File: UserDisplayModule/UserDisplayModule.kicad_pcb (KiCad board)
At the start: 2 copper layers, 0 parts

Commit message: doubled LEDs + started PCB
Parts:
- added C1: 10µ, Capacitor_SMD:C_0805_2012Metric, F.Cu at (60.5, 129.8)
- added D1: MAINS, LED_SMD:LED_0805_2012Metric, F.Cu at (89.2, 78.9)
- added D10: BAT3, LED_SMD:LED_0805_2012Metric, F.Cu at (93.7, 91.1)
- added D11: BAT8, LED_SMD:LED_0805_2012Metric, F.Cu at (100.0, 41.8)
- added D12: BAT1, LED_SMD:LED_0805_2012Metric, F.Cu at (100.0, 44.9)
- added D13: BAT7, LED_SMD:LED_0805_2012Metric, F.Cu at (100.0, 47.9)
- added D14: BAT1, LED_SMD:LED_0805_2012Metric, F.Cu at (100.0, 51.0)
- added D15: BAT6, LED_SMD:LED_0805_2012Metric, F.Cu at (104.5, 41.8)
- added D16: BAT1, LED_SMD:LED_0805_2012Metric, F.Cu at (104.5, 44.9)
- added D17: BAT5, LED_SMD:LED_0805_2012Metric, F.Cu at (104.5, 47.9)
- added D18: BAT1, LED_SMD:LED_0805_2012Metric, F.Cu at (104.5, 51.0)
- added D19: BAT4, LED_SMD:LED_0805_2012Metric, F.Cu at (108.9, 41.8)
- added D2: MAINS, LED_SMD:LED_0805_2012Metric, F.Cu at (89.2, 82.0)
- added D20: BAT1, LED_SMD:LED_0805_2012Metric, F.Cu at (108.9, 44.9)
- added D21: BAT3, LED_SMD:LED_0805_2012Metric, F.Cu at (108.9, 47.9)
- added D22: BAT1, LED_SMD:LED_0805_2012Metric, F.Cu at (108.9, 51.0)
- added D23: BAT2, LED_SMD:LED_0805_2012Metric, F.Cu at (113.4, 41.8)
- added D24: BAT1, LED_SMD:LED_0805_2012Metric, F.Cu at (113.4, 44.9)
- added D25: BAT1, LED_SMD:LED_0805_2012Metric, F.Cu at (113.4, 47.9)
- added D26: BAT1, LED_SMD:LED_0805_2012Metric, F.Cu at (113.4, 51.0)
- added D27: SEG7, LED_SMD:LED_0805_2012Metric, F.Cu at (208.0, 46.4)
- added D28: BAT1, LED_SMD:LED_0805_2012Metric, F.Cu at (208.0, 49.9)
- added D29: SEG6, LED_SMD:LED_0805_2012Metric, F.Cu at (205.1, 52.4)
- added D3: SOLAR, LED_SMD:LED_0805_2012Metric, F.Cu at (89.2, 85.0)
- added D30: BAT1, LED_SMD:LED_0805_2012Metric, F.Cu at (201.6, 52.4)
- added D31: SEG5, LED_SMD:LED_0805_2012Metric, F.Cu at (192.3, 52.4)
- added D32: BAT1, LED_SMD:LED_0805_2012Metric, F.Cu at (195.8, 52.4)
- added D33: SEG4, LED_SMD:LED_0805_2012Metric, F.Cu at (189.5, 46.4)
- added D34: BAT1, LED_SMD:LED_0805_2012Metric, F.Cu at (189.5, 49.9)
- added D35: SEG3, LED_SMD:LED_0805_2012Metric, F.Cu at (195.8, 43.9)
- added D36: BAT1, LED_SMD:LED_0805_2012Metric, F.Cu at (192.3, 43.9)
- added D37: SEG2, LED_SMD:LED_0805_2012Metric, F.Cu at (205.1, 43.9)
- added D38: BAT1, LED_SMD:LED_0805_2012Metric, F.Cu at (201.6, 43.9)
- added D39: SEG1, LED_SMD:LED_0805_2012Metric, F.Cu at (198.8, 46.4)
- added D4: BATTERY, LED_SMD:LED_0805_2012Metric, F.Cu at (89.2, 88.1)
- added D40: BAT1, LED_SMD:LED_0805_2012Metric, F.Cu at (198.8, 49.9)
- added D41: PTVS5V0Z1USK, Diode_SMD:Nexperia_DSN1608-2_1.6x0.8mm, F.Cu at (52.5, 147.3)
- added D42: COL2, LED_SMD:LED_0805_2012Metric, F.Cu at (98.1, 78.9)
- added D43: BAT3, LED_SMD:LED_0805_2012Metric, F.Cu at (98.1, 82.0)
- added D44: COL1, LED_SMD:LED_0805_2012Metric, F.Cu at (98.1, 85.0)
- added D45: BAT3, LED_SMD:LED_0805_2012Metric, F.Cu at (98.1, 88.1)
- added D46: SEG7, LED_SMD:LED_0805_2012Metric, F.Cu at (208.0, 70.2)
- added D47: BAT1, LED_SMD:LED_0805_2012Metric, F.Cu at (208.0, 73.8)
- added D48: SEG6, LED_SMD:LED_0805_2012Metric, F.Cu at (205.1, 76.3)
- added D49: BAT1, LED_SMD:LED_0805_2012Metric, F.Cu at (201.6, 76.3)
- added D5: BATTERY, LED_SMD:LED_0805_2012Metric, F.Cu at (89.2, 91.1)
- added D50: SEG5, LED_SMD:LED_0805_2012Metric, F.Cu at (192.3, 76.2)
- added D51: BAT1, LED_SMD:LED_0805_2012Metric, F.Cu at (195.8, 76.2)
- added D52: SEG4, LED_SMD:LED_0805_2012Metric, F.Cu at (189.5, 70.2)
- added D53: BAT1, LED_SMD:LED_0805_2012Metric, F.Cu at (189.5, 73.7)
- added D54: SEG3, LED_SMD:LED_0805_2012Metric, F.Cu at (195.8, 67.8)
- added D55: BAT1, LED_SMD:LED_0805_2012Metric, F.Cu at (192.3, 67.8)
- added D56: SEG2, LED_SMD:LED_0805_2012Metric, F.Cu at (205.1, 67.8)
- added D57: BAT1, LED_SMD:LED_0805_2012Metric, F.Cu at (201.6, 67.8)
- added D58: SEG1, LED_SMD:LED_0805_2012Metric, F.Cu at (198.8, 70.2)
- added D59: BAT1, LED_SMD:LED_0805_2012Metric, F.Cu at (198.8, 73.8)
- added D6: BAT7, LED_SMD:LED_0805_2012Metric, F.Cu at (93.7, 78.9)
- added D60: SEG7, LED_SMD:LED_0805_2012Metric, F.Cu at (208.0, 94.2)
- added D61: BAT1, LED_SMD:LED_0805_2012Metric, F.Cu at (208.0, 97.8)
- added D62: SEG6, LED_SMD:LED_0805_2012Metric, F.Cu at (205.1, 100.2)
- added D63: BAT1, LED_SMD:LED_0805_2012Metric, F.Cu at (201.6, 100.2)
- added D64: SEG5, LED_SMD:LED_0805_2012Metric, F.Cu at (192.3, 100.2)
- added D65: BAT1, LED_SMD:LED_0805_2012Metric, F.Cu at (195.8, 100.2)
- added D66: SEG4, LED_SMD:LED_0805_2012Metric, F.Cu at (189.5, 94.2)
- added D67: BAT1, LED_SMD:LED_0805_2012Metric, F.Cu at (189.5, 97.8)
- added D68: SEG3, LED_SMD:LED_0805_2012Metric, F.Cu at (195.8, 91.8)
- added D69: BAT1, LED_SMD:LED_0805_2012Metric, F.Cu at (192.3, 91.8)
- added D7: SYS WARN, LED_SMD:LED_0805_2012Metric, F.Cu at (93.7, 82.0)
- added D70: SEG2, LED_SMD:LED_0805_2012Metric, F.Cu at (205.1, 91.8)
- added D71: BAT1, LED_SMD:LED_0805_2012Metric, F.Cu at (201.6, 91.8)
- added D72: SEG1, LED_SMD:LED_0805_2012Metric, F.Cu at (198.8, 94.2)
- added D73: BAT1, LED_SMD:LED_0805_2012Metric, F.Cu at (198.8, 97.8)
- added D74: SEG7, LED_SMD:LED_0805_2012Metric, F.Cu at (207.7, 115.4)
- added D75: BAT1, LED_SMD:LED_0805_2012Metric, F.Cu at (207.7, 118.9)
- added D76: SEG6, LED_SMD:LED_0805_2012Metric, F.Cu at (204.8, 121.5)
- added D77: BAT1, LED_SMD:LED_0805_2012Metric, F.Cu at (201.2, 121.5)
- added D78: SEG5, LED_SMD:LED_0805_2012Metric, F.Cu at (192.0, 121.5)
- added D79: BAT1, LED_SMD:LED_0805_2012Metric, F.Cu at (195.5, 121.5)
- added D8: BAT5, LED_SMD:LED_0805_2012Metric, F.Cu at (93.7, 85.0)
- added D80: SEG4, LED_SMD:LED_0805_2012Metric, F.Cu at (189.2, 115.4)
- added D81: BAT1, LED_SMD:LED_0805_2012Metric, F.Cu at (189.2, 118.9)
- added D82: SEG3, LED_SMD:LED_0805_2012Metric, F.Cu at (195.5, 113.0)
- added D83: BAT1, LED_SMD:LED_0805_2012Metric, F.Cu at (192.0, 113.0)
- added D84: SEG2, LED_SMD:LED_0805_2012Metric, F.Cu at (204.8, 113.0)
- added D85: BAT1, LED_SMD:LED_0805_2012Metric, F.Cu at (201.3, 113.0)
- added D86: SEG1, LED_SMD:LED_0805_2012Metric, F.Cu at (198.4, 115.5)
- added D87: BAT1, LED_SMD:LED_0805_2012Metric, F.Cu at (198.4, 119.0)
- added D9: SYS FAIL, LED_SMD:LED_0805_2012Metric, F.Cu at (93.7, 88.1)
- added H1: MountingHole_Pad, MountingHole:MountingHole_3.2mm_M3_Pad, F.Cu at (32.5, 32.5)
- added H2: MountingHole_Pad, MountingHole:MountingHole_3.2mm_M3_Pad, F.Cu at (32.5, 156.5)
- added H3: MountingHole_Pad, MountingHole:MountingHole_3.2mm_M3_Pad, F.Cu at (220.5, 32.5)
- added H4: MountingHole_Pad, MountingHole:MountingHole_3.2mm_M3_Pad, F.Cu at (220.5, 156.5)
- added J1: RJ45_Shielded, Connector_RJ:RJ45_Shielded_EthernetJack, F.Cu at (48.7, 32.5)
- added R1: R_US, Resistor_SMD:R_0805_2012Metric, F.Cu at (84.8, 78.9)
- added R10: R_US, Resistor_SMD:R_0805_2012Metric, F.Cu at (85.0, 56.6)
- added R11: R_US, Resistor_SMD:R_0805_2012Metric, F.Cu at (85.0, 59.5)
- added R12: R_US, Resistor_SMD:R_0805_2012Metric, F.Cu at (85.0, 62.5)
- added R13: R_US, Resistor_SMD:R_0805_2012Metric, F.Cu at (179.1, 40.1)
- added R14: R_US, Resistor_SMD:R_0805_2012Metric, F.Cu at (179.1, 43.0)
- added R15: R_US, Resistor_SMD:R_0805_2012Metric, F.Cu at (179.1, 46.0)
- added R16: R_US, Resistor_SMD:R_0805_2012Metric, F.Cu at (179.1, 49.0)
- added R17: R_US, Resistor_SMD:R_0805_2012Metric, F.Cu at (179.1, 51.9)
- added R18: R_US, Resistor_SMD:R_0805_2012Metric, F.Cu at (179.1, 54.9)
- added R19: R_US, Resistor_SMD:R_0805_2012Metric, F.Cu at (179.1, 57.8)
- added R2: R_US, Resistor_SMD:R_0805_2012Metric, F.Cu at (84.8, 81.9)
- added R20: R_US, Resistor_SMD:R_0805_2012Metric, F.Cu at (84.8, 90.7)
- added R21: R_US, Resistor_SMD:R_0805_2012Metric, F.Cu at (84.8, 93.7)
- added R22: 16k, Resistor_SMD:R_0805_2012Metric, F.Cu at (56.1, 129.8)
- added R23: R_US, Resistor_SMD:R_0805_2012Metric, F.Cu at (84.8, 96.6)
- added R24: R_US, Resistor_SMD:R_0805_2012Metric, F.Cu at (178.7, 63.6)
- added R25: R_US, Resistor_SMD:R_0805_2012Metric, F.Cu at (178.7, 66.5)
- added R26: R_US, Resistor_SMD:R_0805_2012Metric, F.Cu at (178.7, 69.5)
- added R27: R_US, Resistor_SMD:R_0805_2012Metric, F.Cu at (178.7, 72.4)
- added R28: R_US, Resistor_SMD:R_0805_2012Metric, F.Cu at (178.7, 75.4)
- added R29: R_US, Resistor_SMD:R_0805_2012Metric, F.Cu at (178.7, 78.3)
- added R3: R_US, Resistor_SMD:R_0805_2012Metric, F.Cu at (84.8, 84.8)
- added R30: R_US, Resistor_SMD:R_0805_2012Metric, F.Cu at (178.7, 81.3)
- added R31: R_US, Resistor_SMD:R_0805_2012Metric, F.Cu at (178.9, 87.4)
- added R32: R_US, Resistor_SMD:R_0805_2012Metric, F.Cu at (178.9, 90.4)
- added R33: R_US, Resistor_SMD:R_0805_2012Metric, F.Cu at (178.9, 93.3)
- added R34: R_US, Resistor_SMD:R_0805_2012Metric, F.Cu at (178.9, 96.3)
- added R35: R_US, Resistor_SMD:R_0805_2012Metric, F.Cu at (178.9, 99.2)
- added R36: R_US, Resistor_SMD:R_0805_2012Metric, F.Cu at (178.9, 102.2)
- added R37: R_US, Resistor_SMD:R_0805_2012Metric, F.Cu at (178.9, 105.1)
- added R38: R_US, Resistor_SMD:R_0805_2012Metric, F.Cu at (178.9, 113.1)
- added R39: R_US, Resistor_SMD:R_0805_2012Metric, F.Cu at (178.9, 116.0)
- added R4: R_US, Resistor_SMD:R_0805_2012Metric, F.Cu at (84.8, 87.8)
- added R40: R_US, Resistor_SMD:R_0805_2012Metric, F.Cu at (178.9, 119.0)
- added R41: R_US, Resistor_SMD:R_0805_2012Metric, F.Cu at (178.9, 121.9)
- added R42: R_US, Resistor_SMD:R_0805_2012Metric, F.Cu at (178.9, 124.9)
- added R43: R_US, Resistor_SMD:R_0805_2012Metric, F.Cu at (178.9, 127.8)
- added R44: R_US, Resistor_SMD:R_0805_2012Metric, F.Cu at (178.9, 130.8)
- added R45: 1M, Resistor_SMD:R_0805_2012Metric, F.Cu at (38.4, 32.5)
- added R46: 1M, Resistor_SMD:R_0805_2012Metric, F.Cu at (38.5, 156.5)
- added R47: 1M, Resistor_SMD:R_0805_2012Metric, F.Cu at (214.5, 32.5)
- added R48: 1M, Resistor_SMD:R_0805_2012Metric, F.Cu at (214.4, 156.5)
- added R5: R_US, Resistor_SMD:R_0805_2012Metric, F.Cu at (85.0, 41.8)
- added R6: R_US, Resistor_SMD:R_0805_2012Metric, F.Cu at (85.0, 44.8)
- added R7: R_US, Resistor_SMD:R_0805_2012Metric, F.Cu at (85.0, 47.7)
- added R8: R_US, Resistor_SMD:R_0805_2012Metric, F.Cu at (85.0, 50.7)
- added R9: R_US, Resistor_SMD:R_0805_2012Metric, F.Cu at (85.0, 53.6)
- added RV1: 10K, Potentiometer_THT:Potentiometer_Rotary, F.Cu at (51.5, 141.5)
- added U1: 74HC595, ImportedFootprints:CD74HC595E, F.Cu at (81.1, 97.0)
- added U2: LM324, ImportedFootprints:LM324N, F.Cu at (54.5, 121.8)
- added U3: 74HC595, ImportedFootprints:CD74HC595E, F.Cu at (167.5, 63.5)
- added U4: 74HC595, ImportedFootprints:CD74HC595E, F.Cu at (167.5, 38.5)
- added U5: 74HC595, ImportedFootprints:CD74HC595E, F.Cu at (96.3, 59.9)
- added U6: 74HC595, ImportedFootprints:CD74HC595E, F.Cu at (167.6, 87.7)
- added U7: 74HC595, ImportedFootprints:CD74HC595E, F.Cu at (167.5, 111.3)
- added U8: LM7805_TO220, Package_TO_SOT_THT:TO-220-3_Vertical, F.Cu at (51.0, 53.4)
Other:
- board outline added: 203 x 139 mm

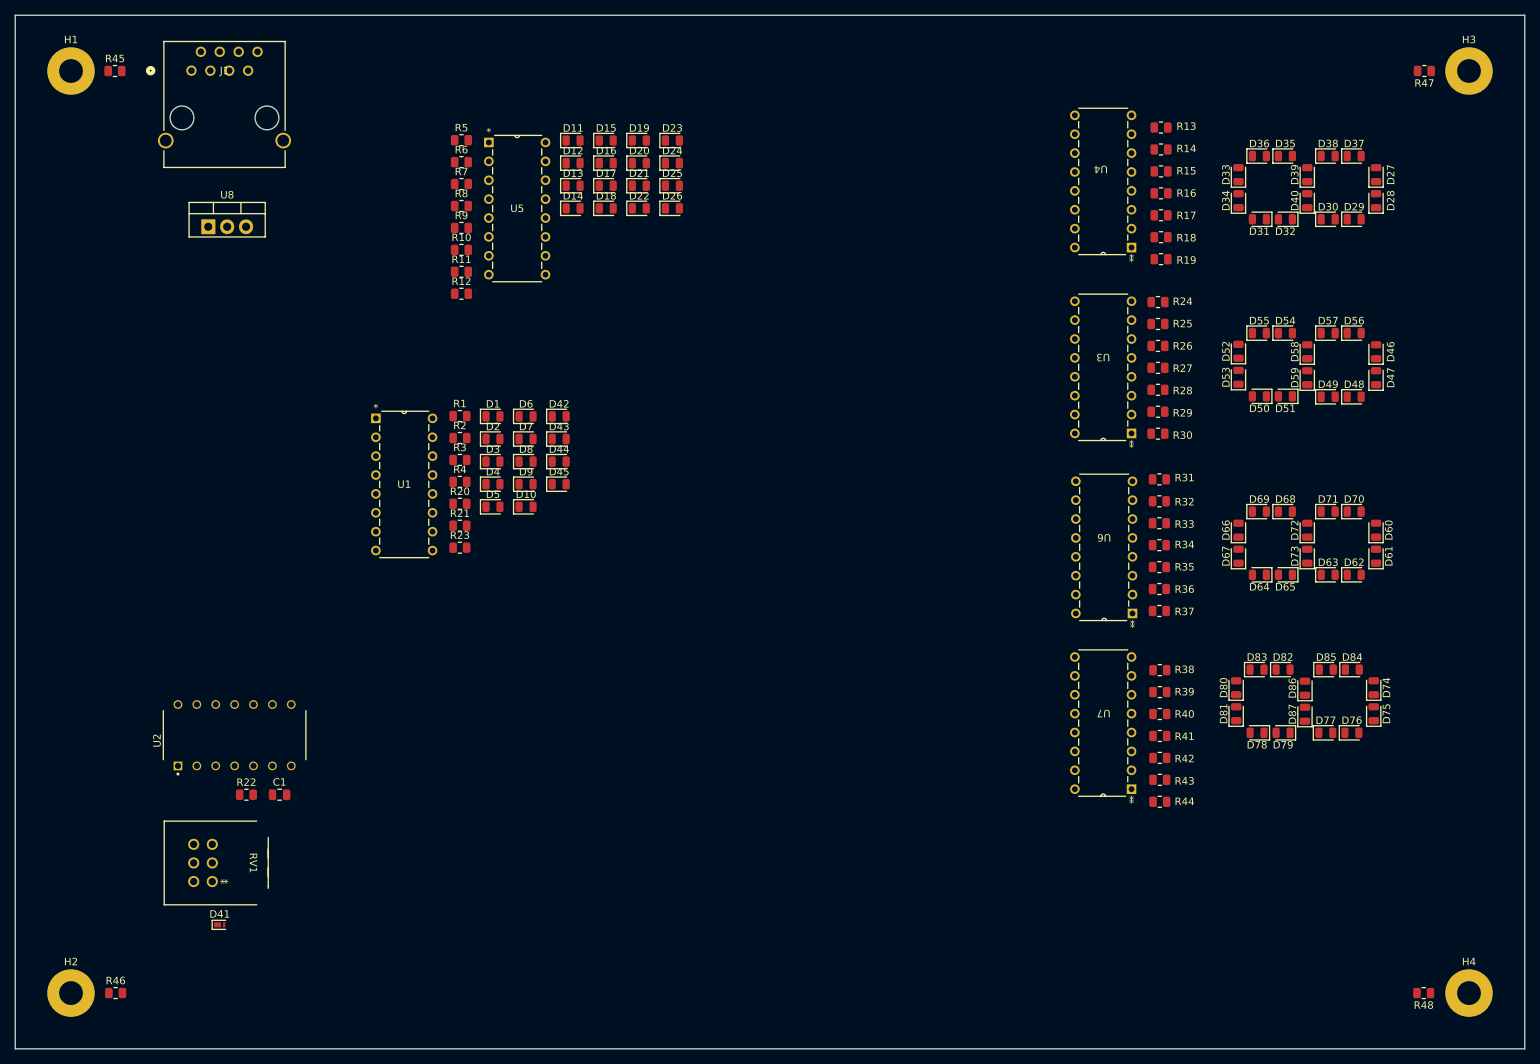
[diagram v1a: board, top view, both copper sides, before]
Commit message: started routing (help)
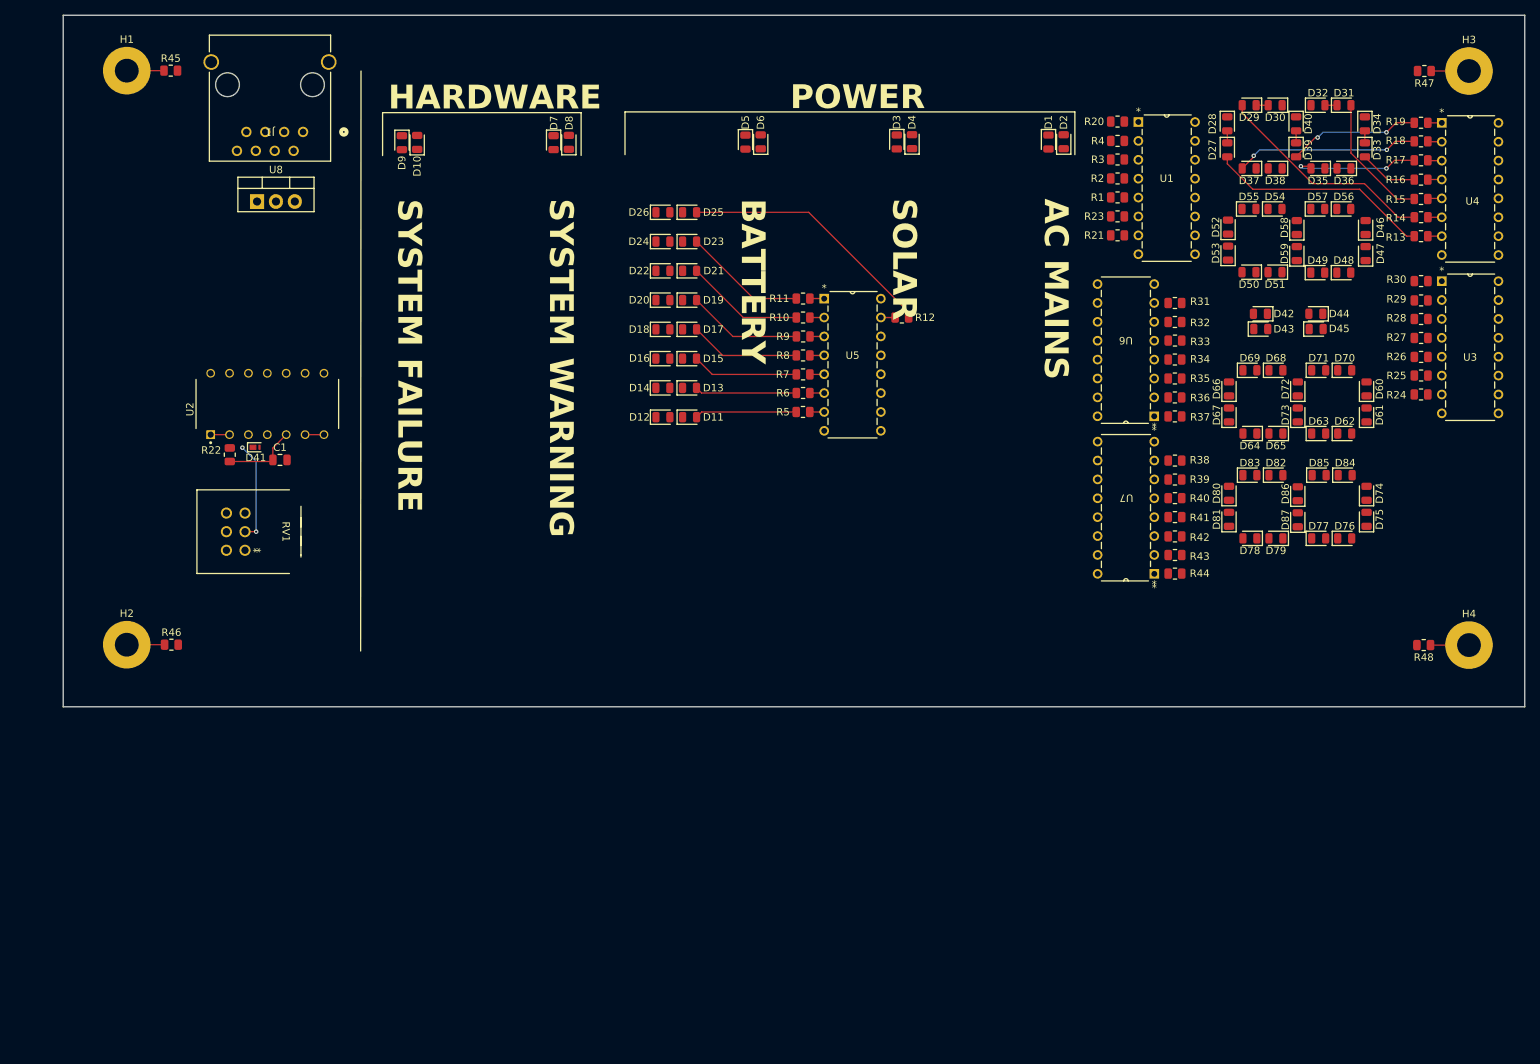
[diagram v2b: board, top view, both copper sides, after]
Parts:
- moved U1 110.0 mm to (183.7, 57.1)
- moved D45 103.9 mm to (200.0, 67.2)
- moved D44 103.7 mm to (199.9, 65.2), turned to 180 degrees
- moved R20 102.3 mm to (173.2, 39.3), turned to 180 degrees
- moved R4 99.6 mm to (173.2, 41.9), turned to 180 degrees
- moved R23 99.0 mm to (173.2, 52.0), turned to 180 degrees
- moved R3 97.2 mm to (173.2, 44.4), turned to 180 degrees
- moved R21 96.7 mm to (173.2, 54.6), turned to 180 degrees
- moved D43 95.5 mm to (192.5, 67.2)
- moved D42 95.3 mm to (192.5, 65.2), turned to 180 degrees
- moved R2 95.1 mm to (173.2, 47.0), turned to 180 degrees
- moved R1 93.2 mm to (173.2, 49.5), turned to 180 degrees
- moved D2 86.5 mm to (166.0, 42.0), turned to 90 degrees
- moved D1 83.3 mm to (163.9, 42.0), turned to -90 degrees
- moved D4 72.8 mm to (145.6, 42.0), turned to 90 degrees
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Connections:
- R1 pad 1: Net-(U1-QH) -> Net-(U1-QF)
- R2 pad 1: Net-(U1-QG) -> Net-(U1-QE)
- R20 pad 1: Net-(U1-QD) -> Net-(U1-QB)
- R21 pad 1: Net-(U1-QC) -> Net-(U1-QH)
- R23 pad 1: Net-(U1-QB) -> Net-(U1-QG)
- R3 pad 1: Net-(U1-QF) -> Net-(U1-QD)
- R4 pad 1: Net-(U1-QE) -> Net-(U1-QC)
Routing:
- net Net-(D25-A): track 0.00 -> 34.8 mm
- net Net-(D27-A): track 0.00 -> 30.1 mm
- net Net-(D29-A): track 0.00 -> 30.0 mm
- net Net-(D37-A): track 0.00 -> 24.7 mm, vias 0 -> 2
- net Net-(D39-A): track 0.00 -> 17.8 mm, vias 0 -> 2
- net Net-(D31-A): track 0.00 -> 17.5 mm
- net Net-(D35-A): track 0.00 -> 17.3 mm, vias 0 -> 2
- net Net-(D23-A): track 0.00 -> 16.6 mm
- net Net-(D21-A): track 0.00 -> 16.0 mm
- net Net-(D19-A): track 0.00 -> 15.5 mm
- net Net-(D17-A): track 0.00 -> 14.9 mm
- net Net-(D15-A): track 0.00 -> 14.3 mm
- net Net-(D13-A): track 0.00 -> 13.7 mm
- net Net-(D11-A): track 0.00 -> 13.7 mm
- net (no net): track 0.00 -> 13.6 mm, vias 0 -> 2
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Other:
- board size 203 x 139 mm -> 196.6 x 93 mm
- board text added: "AC MAINS"
- board text added: "BATTERY"
- board text added: "HARDWARE"
- board text added: "POWER"
- board text added: "SOLAR"
- board text added: "SYSTEM FAILURE"
- board text added: "SYSTEM WARNING"
